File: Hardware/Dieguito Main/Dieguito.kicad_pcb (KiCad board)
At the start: 2 copper layers, 124.4 x 79.8 mm, 46 parts, among them J1 XT30, J2 Cable_PAD, J3 Cable_PAD, J4 Programador, J5 Sensores, J6 Turbina, Q1 AO3400A, SW4 SW_SPDT, U1 ROB-14450, U2 ESP32-WROOM-32, U3 AMS1117-3.3, U4 Mini360

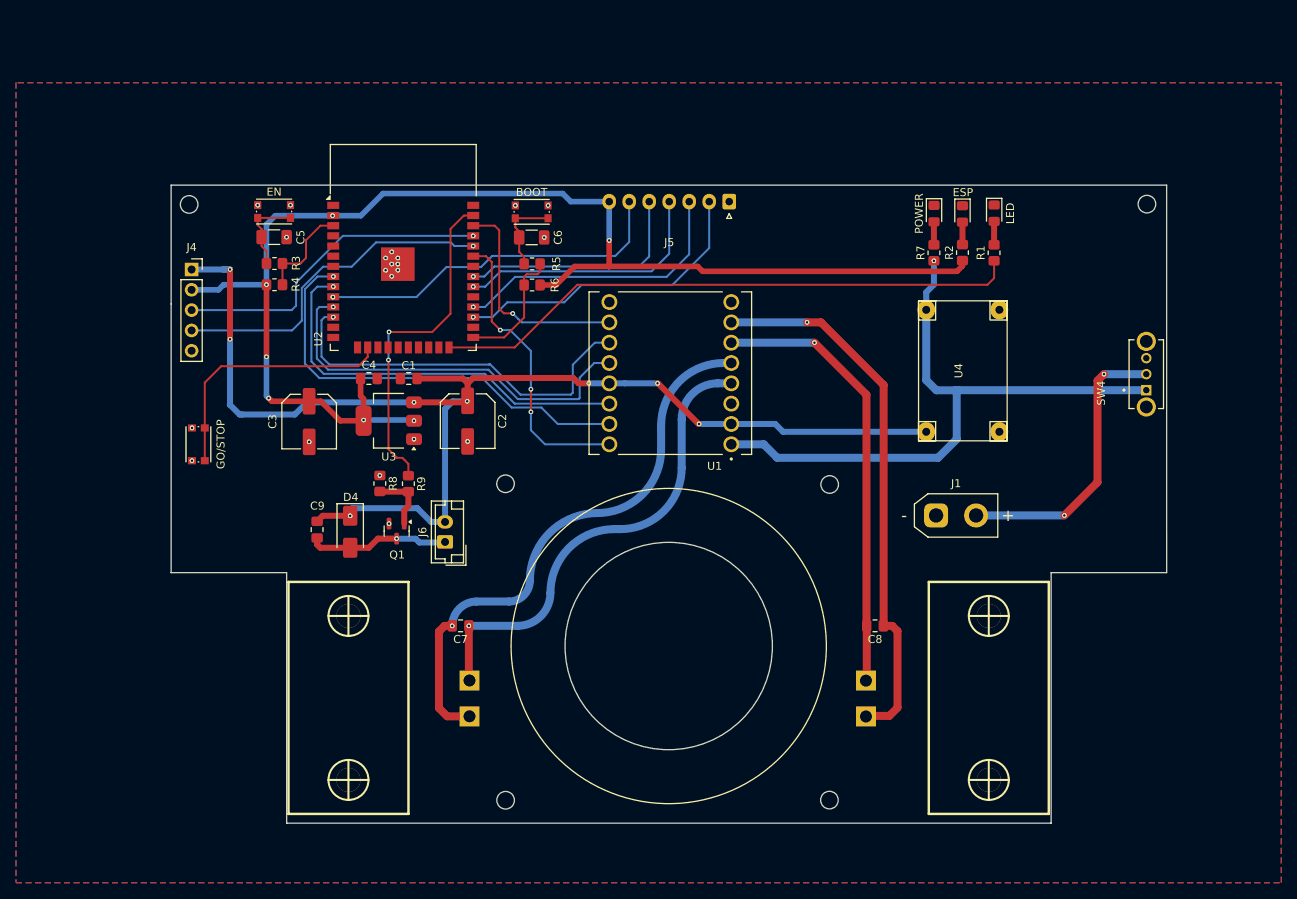
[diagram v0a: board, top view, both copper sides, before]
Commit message: Correcion de placa
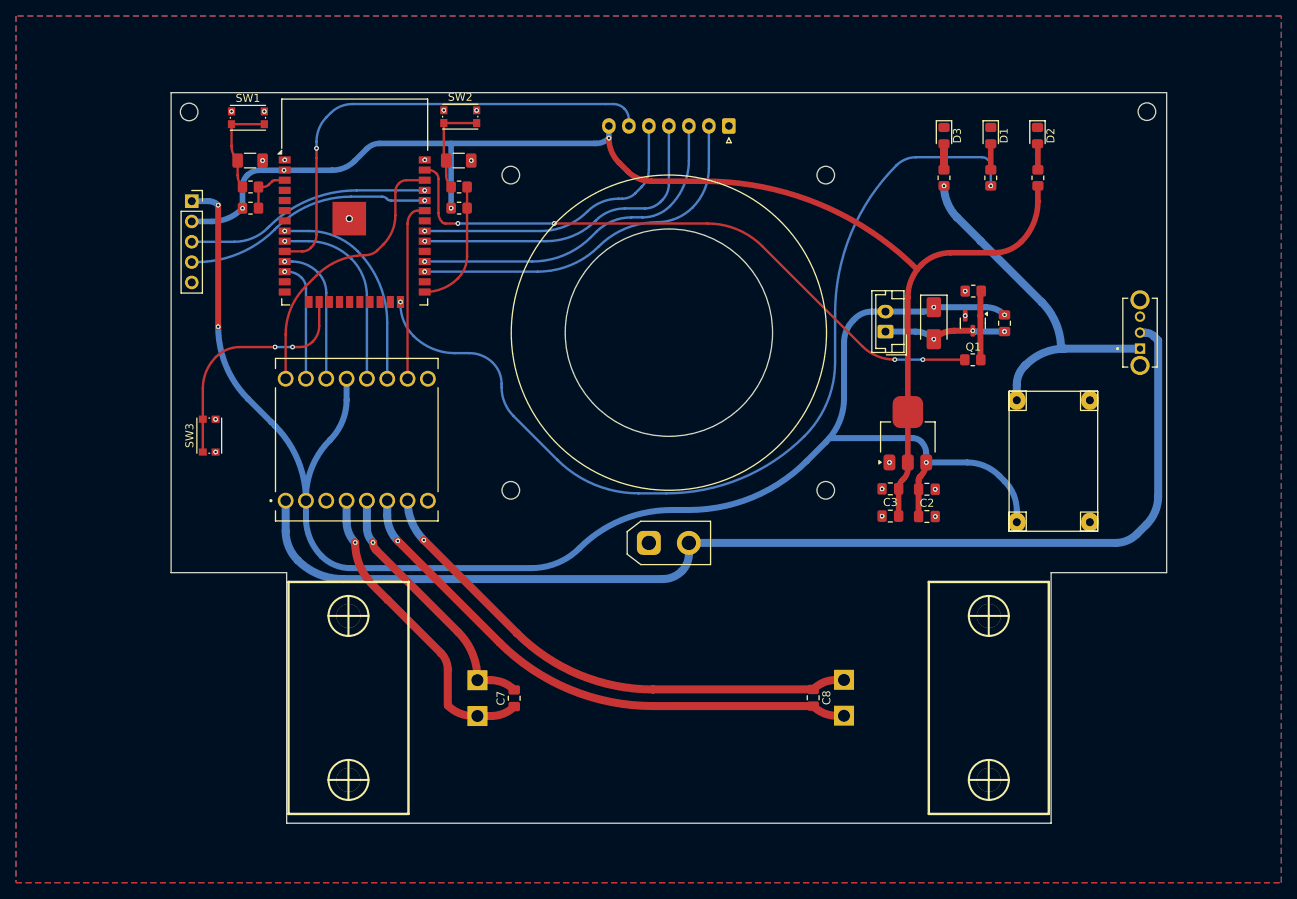
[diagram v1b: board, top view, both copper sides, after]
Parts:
- removed BOOT: BOOT, Button_Switch_SMD:SW_Push_1P1T_NO_CK_KMR2
- removed EN: ENABLE, Button_Switch_SMD:SW_Push_1P1T_NO_CK_KMR2
- removed ESP, LED, POWER: POWER, LED_SMD:LED_0805_2012Metric_Pad1.15x1.40mm_HandSolder
- removed GO/STOP: GO/STOP, Button_Switch_SMD:SW_Push_1P1T_NO_CK_KMR2
- added D1: POWER, LED_SMD:LED_0805_2012Metric_Pad1.15x1.40mm_HandSolder, F.Cu at (250.8, 104.7)
- added D2: POWER, LED_SMD:LED_0805_2012Metric_Pad1.15x1.40mm_HandSolder, F.Cu at (256.6, 104.7)
- added D3: POWER, LED_SMD:LED_0805_2012Metric_Pad1.15x1.40mm_HandSolder, F.Cu at (245.0, 104.7)
- added SW1: ENABLE, Button_Switch_SMD:SW_Push_1P1T_NO_CK_KMR2, F.Cu at (157.9, 102.5)
- added SW2: BOOT, Button_Switch_SMD:SW_Push_1P1T_NO_CK_KMR2, F.Cu at (184.5, 102.3)
- added SW3: GO/STOP, Button_Switch_SMD:SW_Push_1P1T_NO_CK_KMR2, F.Cu at (153.1, 142.2)
- C2, C3: value 100u -> 10u; footprint Capacitor_SMD:C_Elec_6.3x7.7 -> Capacitor_SMD:C_0805_2012Metric_Pad1.18x1.45mm_HandSolder
- moved C9 89.7 mm to (252.5, 128.1)
- moved R8 78.0 mm to (248.6, 124.1), turned to 0 degrees
- moved D4 77.5 mm to (243.7, 128.1)
- moved Q1 76.6 mm to (248.6, 128.1)
- moved C3 73.1 mm to (238.3, 148.8), turned to 180 degrees
- moved R9 72.2 mm to (248.6, 132.7), turned to 180 degrees
- moved C4 67.4 mm to (238.3, 152.2), turned to 180 degrees
- moved C1 66.2 mm to (242.8, 148.9), turned to 0 degrees
- moved U3 64.9 mm to (240.4, 142.4), turned to 90 degrees
- moved J6 61.0 mm to (237.6, 129.2)
- moved C2 58.6 mm to (242.8, 152.3), turned to 0 degrees
- moved REF** 55.6 mm to (230.2, 109.6)
- moved REF** 55.5 mm to (190.8, 109.6)
- moved U1 40.1 mm to (171.6, 142.7), turned to 90 degrees
- moved REF** 38.7 mm to (190.8, 149.0)
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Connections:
- J1 pad 2: Net-(J1-Pin_2) -> /VM
- J2 pad 1: Net-(U1-A01) -> Net-(U1-A02)
- J2 pad 2: Net-(U1-A02) -> Net-(U1-A01)
- J3 pad 1: Net-(U1-B01) -> Net-(U1-B02)
- J3 pad 2: Net-(U1-B02) -> Net-(U1-B01)
- SW4 pad 2: Net-(J1-Pin_2) -> /VM
- U1 pad 1: VCC -> /VM
- U2 pad 11: BI1 -> AI1
- U2 pad 12: BI2 -> AI2
- U2 pad 33: PWMA -> PWMB
- U2 pad 36: PWMB -> PWMA
- U2 pad 8: AI2 -> BI2
- U2 pad 9: AI1 -> BI1
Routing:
- net /VM: track 0.00 -> 144.4 mm
- net +5V: track 157.8 -> 208.5 mm, vias 8 -> 5
- net LED: track 73.9 -> 116.0 mm, vias 0 -> 2
- net AI2: track 54.7 -> 15.1 mm
- net D23: track 42.2 -> 79.6 mm, vias 2 -> 4
- net Net-(U1-A02): track 69.5 -> 32.5 mm
- net Net-(J1-Pin_2): track 36.0 -> 0.00 mm, vias 2 -> 0
- net VCC: track 79.3 -> 45.3 mm
- net AI1: track 51.1 -> 18.0 mm
- net BI1: track 50.3 -> 24.4 mm
- net BI2: track 48.9 -> 26.6 mm
- net Net-(U1-A01): track 58.6 -> 39.1 mm
- net SIG: track 44.7 -> 60.4 mm
- net Net-(U1-B02): track 55.1 -> 68.7 mm
- net RXD0: track 42.3 -> 31.3 mm
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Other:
- board size 124.4 x 79.8 mm -> 124.4 x 91.3 mm
